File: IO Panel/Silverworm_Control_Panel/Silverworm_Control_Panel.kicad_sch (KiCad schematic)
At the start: 30 parts, among them J1 Microfit 6-pin, J2 Conn_01x15, J3 Conn_01x15, J4 JST-PH-2PIN, J5 JST-PH-2PIN, J6 JST-PH-2PIN, J7 JST-PH-2PIN, SW1 SW_SPDT

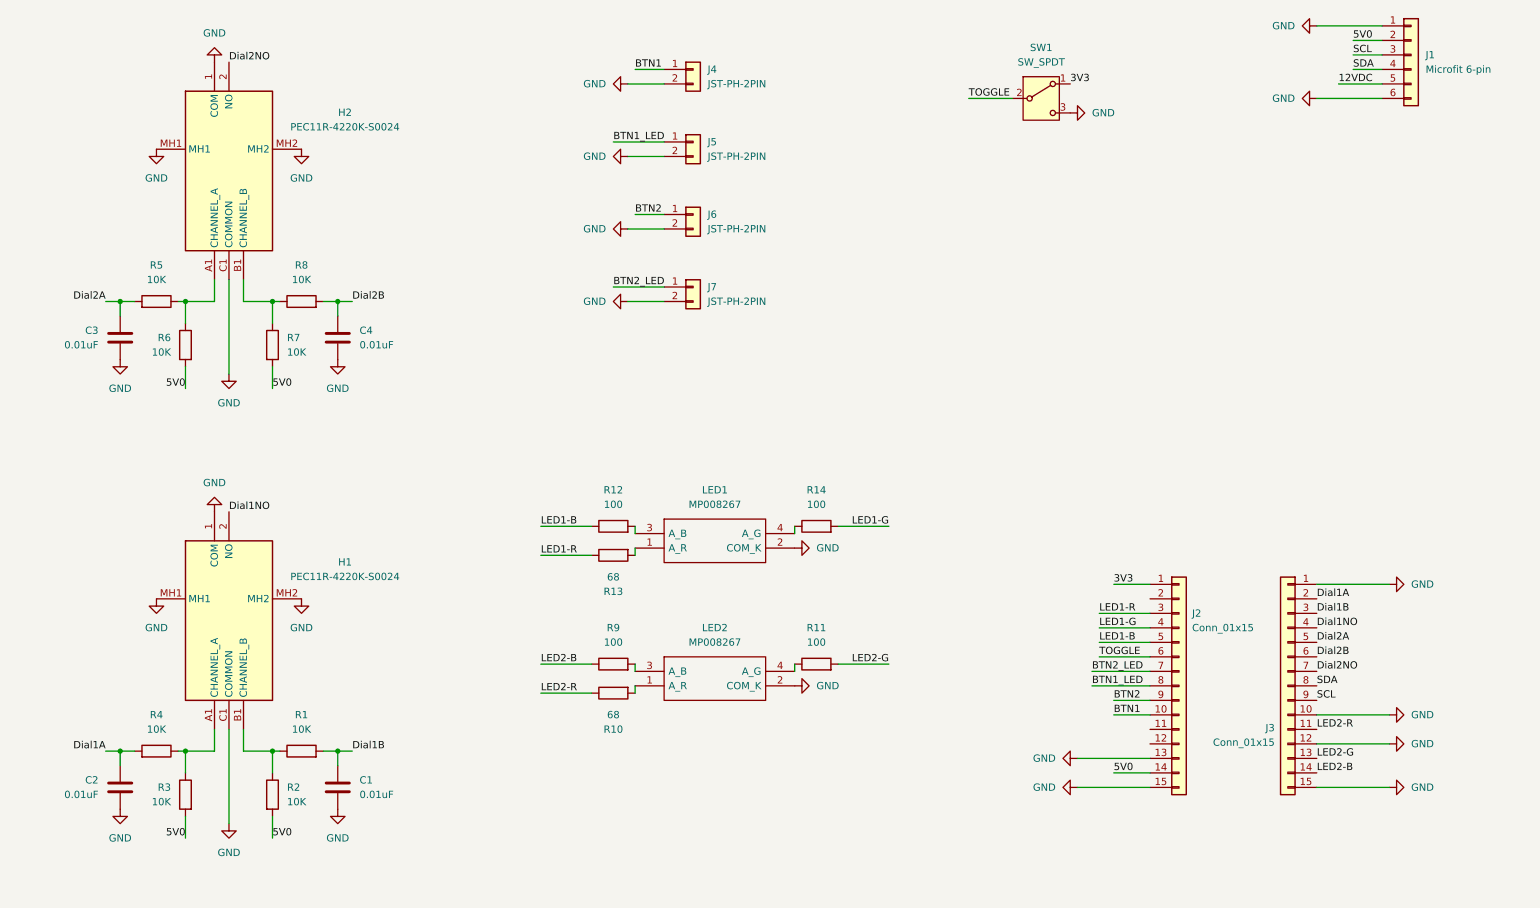
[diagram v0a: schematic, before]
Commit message: Layout and IO edits
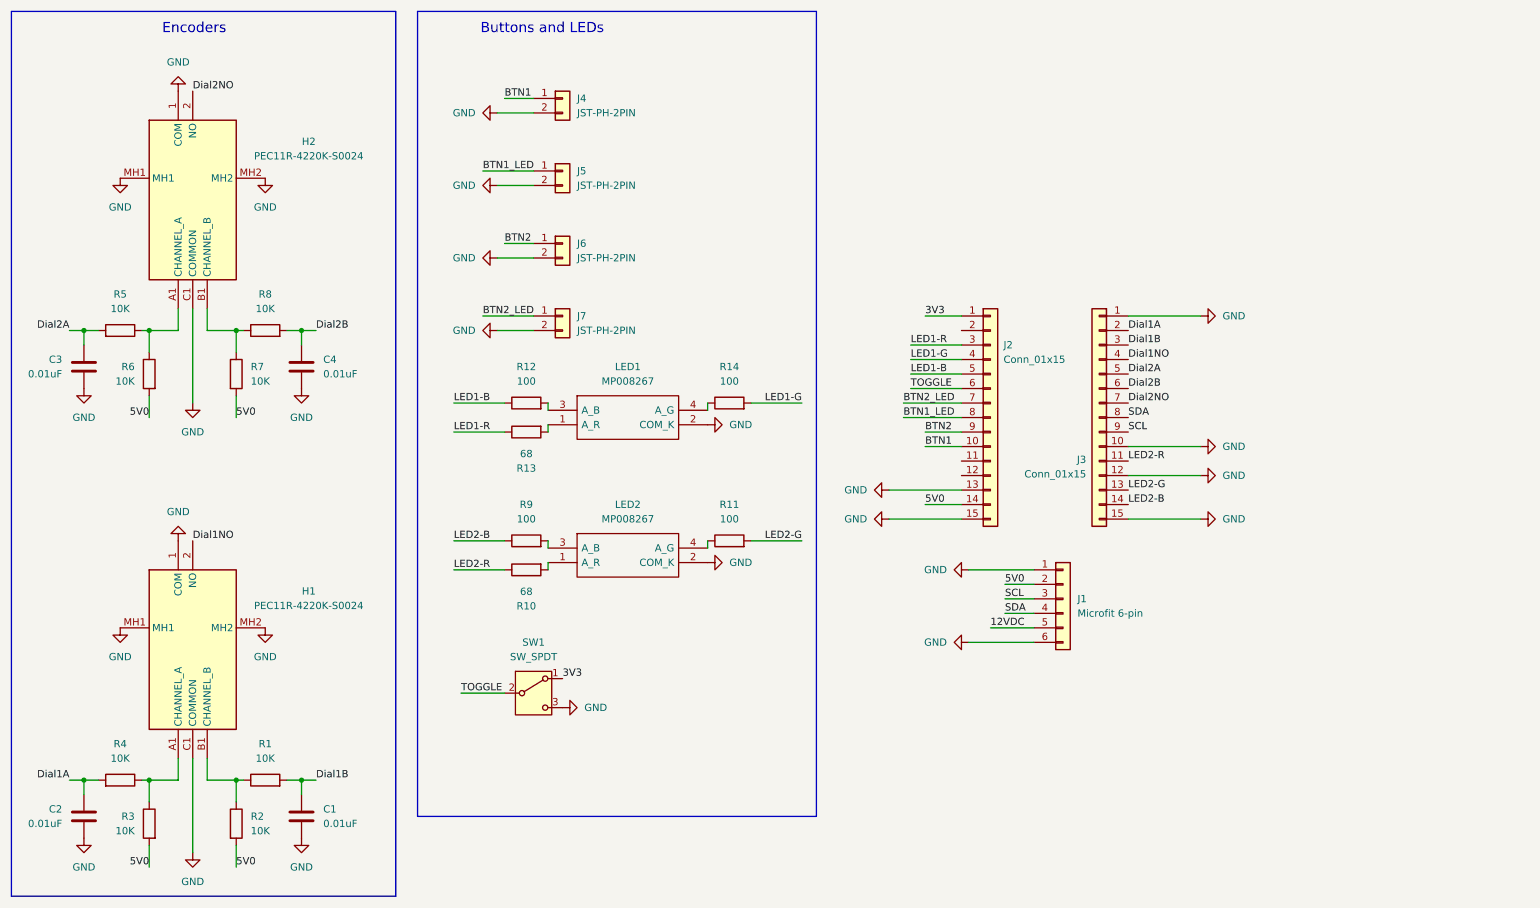
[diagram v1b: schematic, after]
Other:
- note added: "Buttons and LEDs"
- note added: "Encoders"
- moved on the sheet: C1, C2, C3, C4, H1, H2, J1, J2, J3, J4, J5, J6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
